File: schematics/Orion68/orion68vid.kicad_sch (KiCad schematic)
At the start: 27 parts, among them J300 Euro96pin, Q4 2N7000, U301 74HC245, U302 74HC245, U303 24LC256, U304 GAL16V8, U305 74LS541

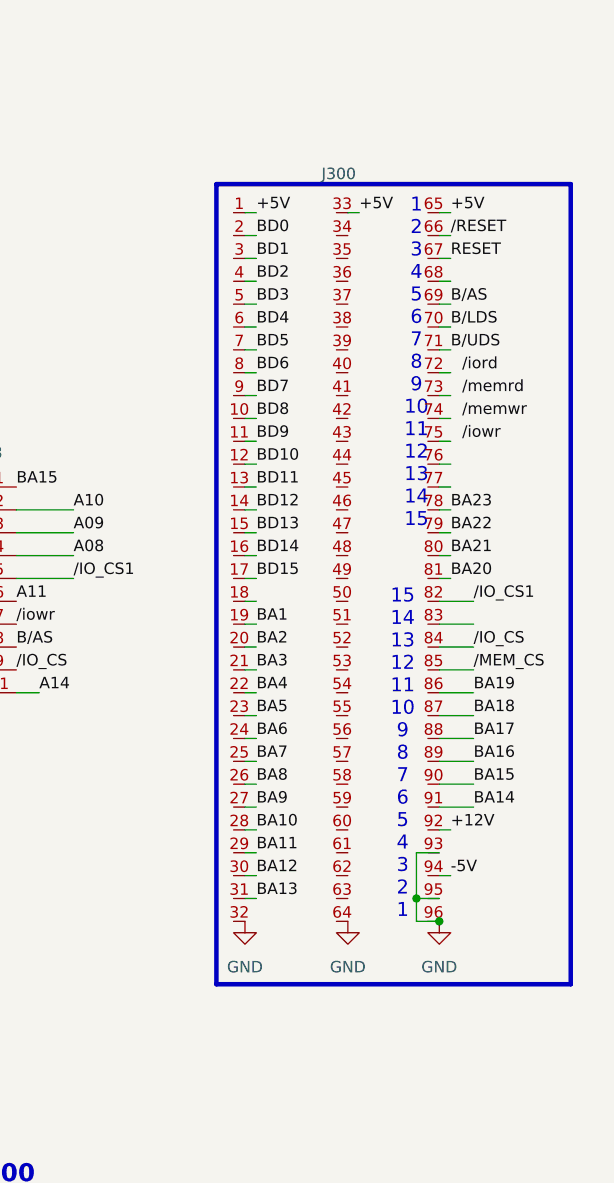
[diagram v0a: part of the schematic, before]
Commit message: update
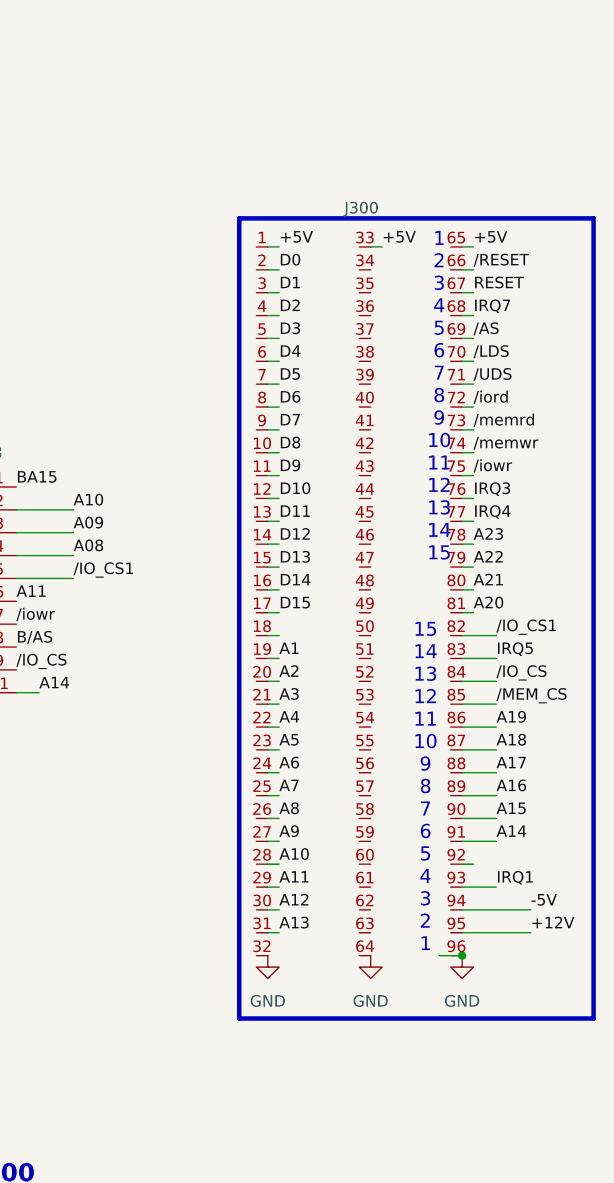
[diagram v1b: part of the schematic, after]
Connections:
- net BA10 is gone; now on net A10: J300.28
- net BA11 is gone; now on net A11: J300.29
- net BA12 is gone; now on net A12: J300.30
- net BA13 is gone; now on net A13: J300.31
- net BA14 is gone; now on net A14: J300.91
- net +12V: now also J300.95; no longer J300.92
- net BA1: no longer J300.19
- net BA15: no longer J300.90
- net BA2: no longer J300.20
- net BA3: no longer J300.21
- net BA4: no longer J300.22
- net BA5: no longer J300.23
- net BD0: no longer J300.2
- net BD1: no longer J300.3
- net BD2: no longer J300.4
- net BD3: no longer J300.5
- net BD4: no longer J300.6
- net BD5: no longer J300.7
- net BD6: no longer J300.8
- net BD7: no longer J300.9
- net B/AS: no longer J300.69
- net D0: now also J300.2
- net D1: now also J300.3
- net D2: now also J300.4
- net D3: now also J300.5
- net D4: now also J300.6
- net D5: now also J300.7
- net D6: now also J300.8
- net D7: now also J300.9
- net GND: no longer J300.93, J300.95
- net /iord: now also J300.72
- net /iowr: now also J300.75
- net /memrd: now also J300.73
- net /memwr: now also J300.74
- net IRQ7: now reaches J300.68
- net IRQ3: now reaches J300.76
- net IRQ4: now reaches J300.77
- net IRQ5: now reaches J300.83
- net BA16 renamed A16
- net BA17 renamed A17
- net BA18 renamed A18
- net BA19 renamed A19
- net BA20 renamed A20
- net BA21 renamed A21
- net BA22 renamed A22
- net BA23 renamed A23
- net BA6 renamed A6
- net BA7 renamed A7
- net BA8 renamed A8
- net BA9 renamed A9
- net BD10 renamed D10
- net BD11 renamed D11
- net BD12 renamed D12
- net BD13 renamed D13
- net BD14 renamed D14
- net BD15 renamed D15
- net BD8 renamed D8
- net BD9 renamed D9
- net B/LDS renamed /LDS
- net B/UDS renamed /UDS
- new net A1: J300.19
- new net A15: J300.90
- new net A2: J300.20
- new net A3: J300.21
- new net A4: J300.22
- new net A5: J300.23
- new net IRQ1: J300.93
- new net /AS: J300.69
